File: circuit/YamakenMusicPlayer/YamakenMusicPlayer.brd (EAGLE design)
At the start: 100 x 80 mm, 24 parts, among them J1 DCJ0202, J2 AJ-1780, U1 NJM2396F33, U2 AE-ESP-WROOM-02

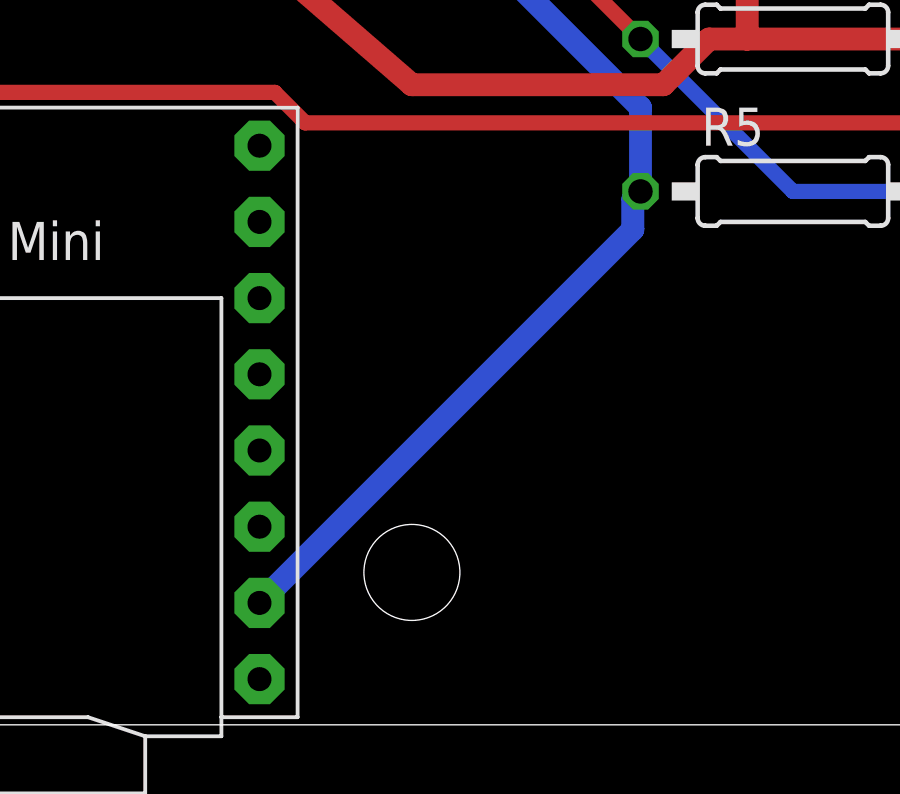
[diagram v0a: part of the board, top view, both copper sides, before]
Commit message: 表記の修正
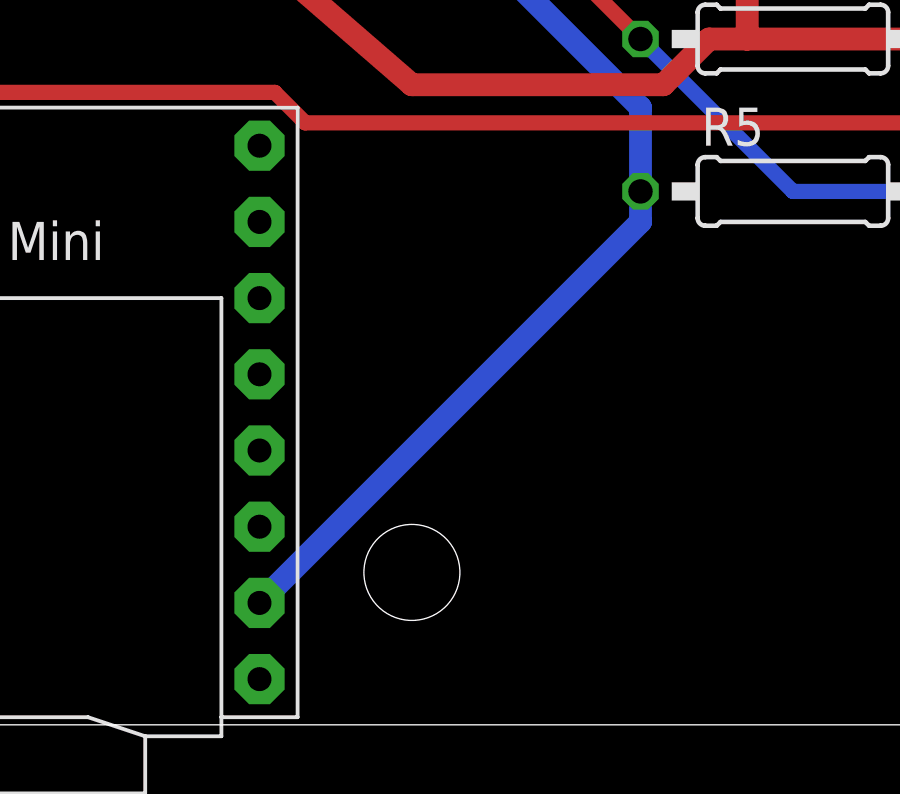
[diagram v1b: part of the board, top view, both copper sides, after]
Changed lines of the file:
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@@
 <contactref element="U2" pad="P13"/>
 <contactref element="U2" pad="P18"/>
-<contactref element="U$1" pad="GND_2"/>
 <wire x1="78.74" y1="8.89" x2="74.676" y2="8.89" width="0.762" layer="16"/>
 <wire x1="74.676" y1="8.89" x2="68.58" y2="8.89" width="0.762" layer="16"/>
@@
 <wire x1="27.94" y1="27.94" x2="27.94" y2="25.4" width="0.762" layer="16"/>
 <wire x1="38.1" y1="38.1" x2="27.94" y2="27.94" width="0.762" layer="16"/>
-<wire x1="53.086" y1="16.51" x2="40.64" y2="4.064" width="0.762" layer="16"/>
-<wire x1="53.086" y1="17.526" x2="53.086" y2="16.51" width="0.762" layer="16"/>
-<wire x1="53.086" y1="17.526" x2="53.34" y2="17.78" width="0.762" layer="16"/>
 <wire x1="23.114" y1="52.07" x2="23.114" y2="63.246" width="0.762" layer="16"/>
 <wire x1="37.338" y1="37.846" x2="23.114" y2="52.07" width="0.762" layer="16"/>
@@
 <vertex x="55.88" y="40.64"/>
 </polygon>
+<contactref element="U$1" pad="GND_2"/>
+<wire x1="40.64" y1="4.064" x2="53.34" y2="16.764" width="0.762" layer="16"/>
+<wire x1="53.34" y1="16.764" x2="53.34" y2="17.78" width="0.762" layer="16"/>
 </signal>
 <signal name="N$1">
